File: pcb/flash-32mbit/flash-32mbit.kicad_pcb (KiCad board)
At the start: 2 copper layers, 96.3 x 76.2 mm, 33 parts, among them U1 LH28F320SKTD-L70, U2 AS6C1008-55SIN, U3 SN74LVC1G04, U4 RP2040-Tiny, U5 MCP23S17-E/SO, U6 MCP23S17-E/SO, U7 MCP23S17-E/SO

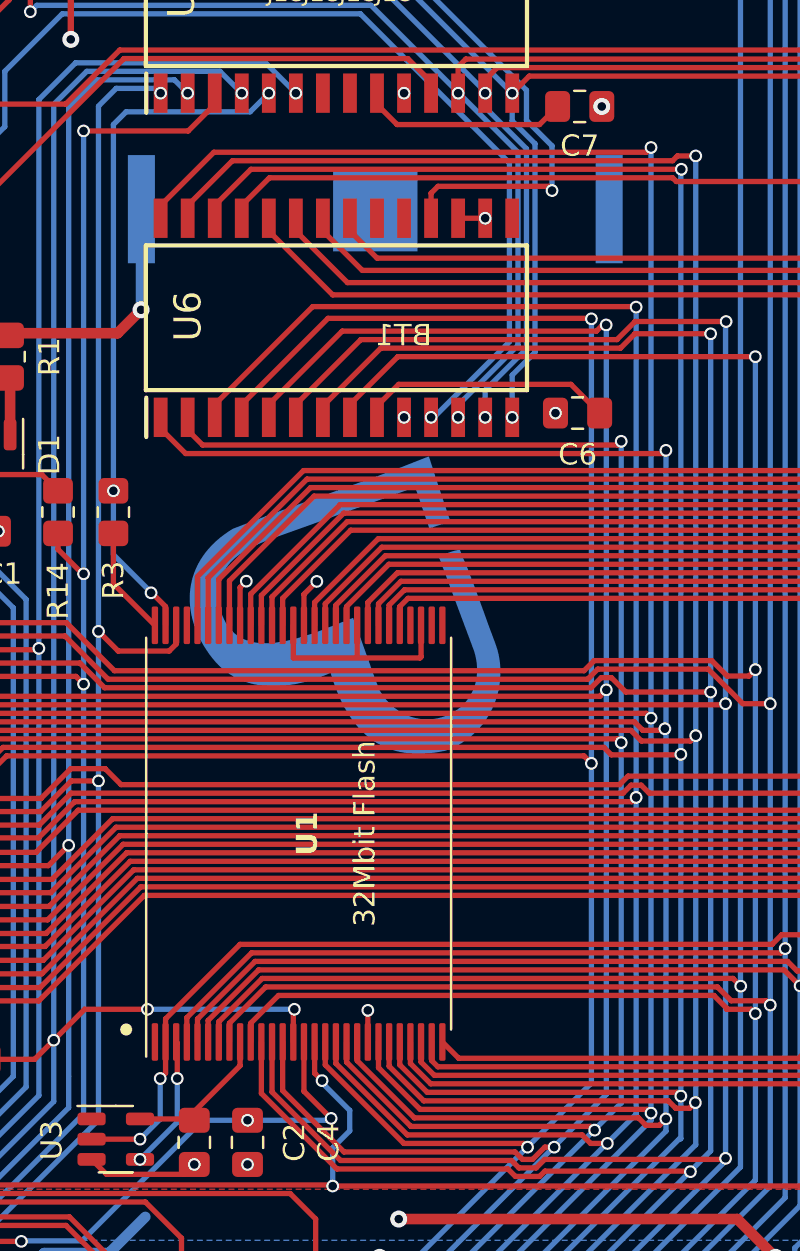
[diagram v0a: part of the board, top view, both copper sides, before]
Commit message: Widens battery solder pads
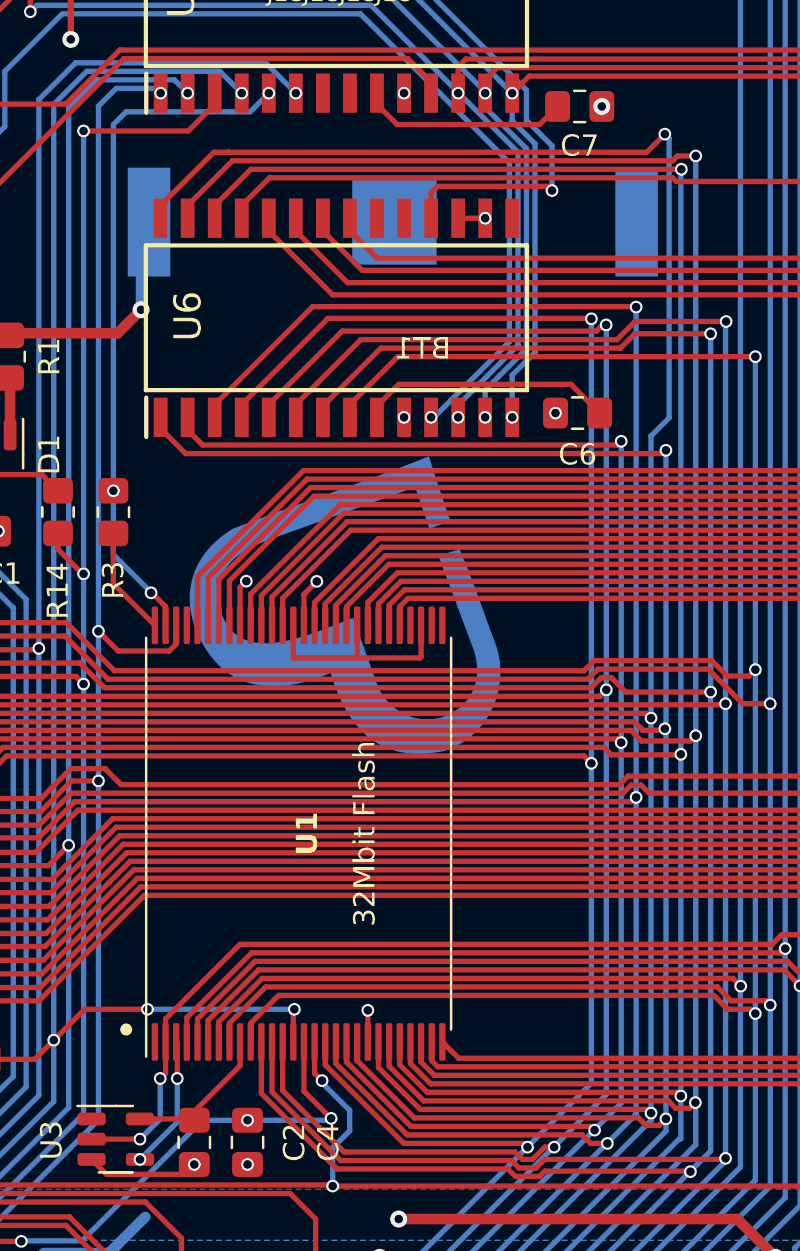
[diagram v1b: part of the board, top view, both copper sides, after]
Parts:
- moved BT1 1.10 mm to (147.6, 77.9)
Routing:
- net +BATT: track 13.0 -> 10.7 mm
- net /A7: track 146.3 -> 148.3 mm
- net GND: track 106.2 -> 104.3 mm
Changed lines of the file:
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@@
   (title_block
     (title "Floopy Drive")
-    (date "2023-12-09")
+    (date "2024-01-16")
     (rev "9")
     (company "@partlyhuman")
@@
   )
   (footprint "LOOPY_Cart:Keystone-3034TR-MFG" (layer "B.Cu")
-    (at 146.7 77.3 180)
+    (at 147.6 77.925 180)
     (property "Notes" "")
     (property "Sheetfile" "flash-32mbit.kicad_sch")
@@
         (effects (font (size 1.27 1.27) (thickness 0.15)) (justify mirror))
     )
-    (fp_line (start -13 -0.67) (end -12 -0.67)
+    (fp_line (start -12.2 3.199999) (end -11.2 3.199999)
       (stroke (width 0.15) (type solid)) (layer "B.SilkS"))
-    (fp_line (start -12.5 -0.169999) (end -12.5 -1.17)
+    (fp_line (start -11.7 3.7) (end -11.7 2.699999)
       (stroke (width 0.15) (type solid)) (layer "B.SilkS"))
     (fp_line (start -10.73 -3.6) (end -10.73 -5.185)
@@
     (fp_line (start 10.73 4.189999) (end 10.73 2.3)
       (stroke (width 0.15) (type solid)) (layer "B.SilkS"))
-    (fp_line (start -11.644999 -8.2165) (end 11.644999 -8.2165)
+    (fp_line (start -12.9 -8.232998) (end 12.7 -8.2)
       (stroke (width 0.15) (type solid)) (layer "B.CrtYd"))
-    (fp_line (start -11.644999 8.216498) (end -11.644999 -8.2165)
+    (fp_line (start -12.9 8.2) (end -12.9 -8.232998)
       (stroke (width 0.15) (type solid)) (layer "B.CrtYd"))
-    (fp_line (start 11.644999 -8.2165) (end 11.644999 8.216498)
+    (fp_line (start 12.7 -8.2) (end 12.7 8.232998)
       (stroke (width 0.15) (type solid)) (layer "B.CrtYd"))
-    (fp_line (start 11.644999 8.216498) (end -11.644999 8.216498)
-      (stroke (width 0.15) (type solid)) (layer "B.CrtYd"))
-    (fp_line (start 11.644999 8.216498) (end 11.644999 8.216498)
+    (fp_line (start 12.7 8.232998) (end -12.9 8.2)
       (stroke (width 0.15) (type solid)) (layer "B.CrtYd"))
     (fp_line (start -10.7315 -8.1915) (end -10.7315 8.191498)
@@
     (fp_line (start 10.7315 8.191498) (end 10.7315 -8.1915)
       (stroke (width 0.15) (type solid)) (layer "B.Fab"))
-    (pad "" smd rect (at -10.984999 -0.673099 180) (size 1.27 5.08) (layers "B.Cu" "B.Paste" "B.Mask"))
-    (pad "1" smd rect (at 10.984999 -0.6731 180) (size 1.27 5.08) (layers "B.Cu" "B.Paste" "B.Mask")
+    (pad "" smd rect (at -11.374999 -0.673098 180) (size 2 5.079998) (layers "B.Cu" "B.Paste" "B.Mask"))
+    (pad "1" smd rect (at 11.524999 -0.65655 180) (size 2 5.1131) (layers "B.Cu" "B.Paste" "B.Mask")
       (net 56 "+BATT") (pinfunction "+") (pintype "passive"))
     (pad "2" smd rect (at 0 -0.673099 180) (size 3.9624 3.9624) (layers "B.Cu" "B.Mask")
@@
   (segment (start 163.831233 61.968767) (end 163.85 61.987534) (width 0.25) (layer "B.Cu") (net 2))
   (segment (start 125.63 101.83) (end 125.005 101.205) (width 0.25) (layer "F.Cu") (net 3))
-  (segment (start 139.119 75.3) (end 136.62 77.799) (width 0.25) (layer "F.Cu") (net 3))
   (segment (start 146.85 117.084) (end 146.85 118.291403) (width 0.25) (layer "F.Cu") (net 3))
-  (segment (start 159.425 75.3) (end 139.119 75.3) (width 0.25) (layer "F.Cu") (net 3))
+  (segment (start 159.4505 75.2995) (end 139.823815 75.2995) (width 0.25) (layer "F.Cu") (net 3))
   (segment (start 146.85 118.291403) (end 148.808598 120.25) (width 0.25) (layer "F.Cu") (net 3))
   (segment (start 159.4245 101.65) (end 128.18 101.65) (width 0.25) (layer "F.Cu") (net 3))
-  (segment (start 159.65 75.075) (end 159.425 75.3) (width 0.25) (layer "F.Cu") (net 3))
   (segment (start 125.005 101.205) (end 113.537 101.205) (width 0.25) (layer "F.Cu") (net 3))
+  (segment (start 139.823815 75.2995) (end 139.823315 75.3) (width 0.25) (layer "F.Cu") (net 3))
   (segment (start 148.808598 120.25) (end 159.4755 120.25) (width 0.25) (layer "F.Cu") (net 3))
+  (segment (start 139.823315 75.3) (end 139.119 75.3) (width 0.25) (layer "F.Cu") (net 3))
   (segment (start 159.65 101.8755) (end 159.4245 101.65) (width 0.25) (layer "F.Cu") (net 3))
-  (segment (start 159.4755 120.25) (end 159.65 120.4245) (width 0.25) (layer "F.Cu") (net 3))
+  (segment (start 139.119 75.3) (end 136.62 77.799) (width 0.25) (layer "F.Cu") (net 3))
   (segment (start 136.62 77.799) (end 136.62 78.399) (width 0.25) (layer "F.Cu") (net 3))
+  (segment (start 159.4755 120.25) (end 159.65 120.4245) (width 0.25) (layer "F.Cu") (net 3))
+  (segment (start 160.3 74.45) (end 159.4505 75.2995) (width 0.25) (layer "F.Cu") (net 3))
   (segment (start 128 101.83) (end 125.63 101.83) (width 0.25) (layer "F.Cu") (net 3))
   (segment (start 128.18 101.65) (end 128 101.83) (width 0.25) (layer "F.Cu") (net 3))
   (via (at 159.65 101.8755) (size 0.6) (drill 0.4) (layers "F.Cu" "B.Cu") (net 3))
   (via (at 159.65 120.4245) (size 0.6) (drill 0.4) (layers "F.Cu" "B.Cu") (net 3))
-  (via (at 159.65 75.075) (size 0.6) (drill 0.4) (layers "F.Cu" "B.Cu") (net 3))
-  (segment (start 159.65 75.075) (end 159.65 120.762563) (width 0.25) (layer "B.Cu") (net 3))
+  (via (at 160.3 74.45) (size 0.6) (drill 0.4) (layers "F.Cu" "B.Cu") (net 3))
+  (segment (start 160.5 87.775) (end 159.65 88.625) (width 0.25) (layer "B.Cu") (net 3))
+  (segment (start 159.65 88.625) (end 159.65 120.762563) (width 0.25) (layer "B.Cu") (net 3))
   (segment (start 152.3 131.9) (end 152.5 132.1) (width 0.25) (layer "B.Cu") (net 3))
+  (segment (start 160.3 74.45) (end 160.5 74.65) (width 0.25) (layer "B.Cu") (net 3))
   (segment (start 152.3 128.112563) (end 152.3 131.9) (width 0.25) (layer "B.Cu") (net 3))
   (segment (start 159.65 120.762563) (end 152.3 128.112563) (width 0.25) (layer "B.Cu") (net 3))
+  (segment (start 160.5 74.65) (end 160.5 87.775) (width 0.25) (layer "B.Cu") (net 3))
   (segment (start 113.537 102.475) (end 124.875 102.475) (width 0.25) (layer "F.Cu") (net 4))
   (segment (start 154.4 129.45) (end 155.5 128.35) (width 0.25) (layer "F.Cu") (net 4))
@@
   (segment (start 164.9 131.9) (end 165.1 132.1) (width 0.5) (layer "B.Cu") (net 16))
   (segment (start 129.7 128.4) (end 129.750579 128.4) (width 0.5) (layer "B.Cu") (net 16))
-  (segment (start 148.05 76.623099) (end 146.7 77.973099) (width 0.5) (layer "B.Cu") (net 16))
   (segment (start 106.32 62.88) (end 106.3 62.9) (width 1) (layer "B.Cu") (net 16))
   (segment (start 165.5 127.2) (end 164.9 127.8) (width 0.5) (layer "B.Cu") (net 16))
@@
   (segment (start 129.6 83.8) (end 134.6 83.8) (width 0.5) (layer "F.Cu") (net 56))
   (via (at 135.7 82.7) (size 0.8) (drill 0.4) (layers "F.Cu" "B.Cu") (net 56))
-  (segment (start 135.7 82.7) (end 135.7 77.988101) (width 0.5) (layer "B.Cu") (net 56))
-  (segment (start 135.7 77.988101) (end 135.715001 77.9731) (width 0.5) (layer "B.Cu") (net 56))
-  (segment (start 135.8 79.5) (end 135.715001 79.415001) (width 0.4) (layer "B.Cu") (net 56))
-  (segment (start 135.715001 79.415001) (end 135.715001 77.9731) (width 0.4) (layer "B.Cu") (net 56))
+  (segment (start 135.7 82.7) (end 135.7 78.738101) (width 0.5) (layer "B.Cu") (net 56))
   (segment (start 120.8 129.1) (end 120.8 131.9) (width 0.25) (layer "F.Cu") (net 61))
   (segment (start 122.6 128.4) (end 121.5 128.4) (width 0.25) (layer "F.Cu") (net 61))
